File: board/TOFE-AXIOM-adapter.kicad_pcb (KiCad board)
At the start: 4 copper layers, 68.9 x 31.9 mm, 21 parts, among them CN1 C, U1 24AA01/24LC01B, U2 LM317T, U3 LM7805CT

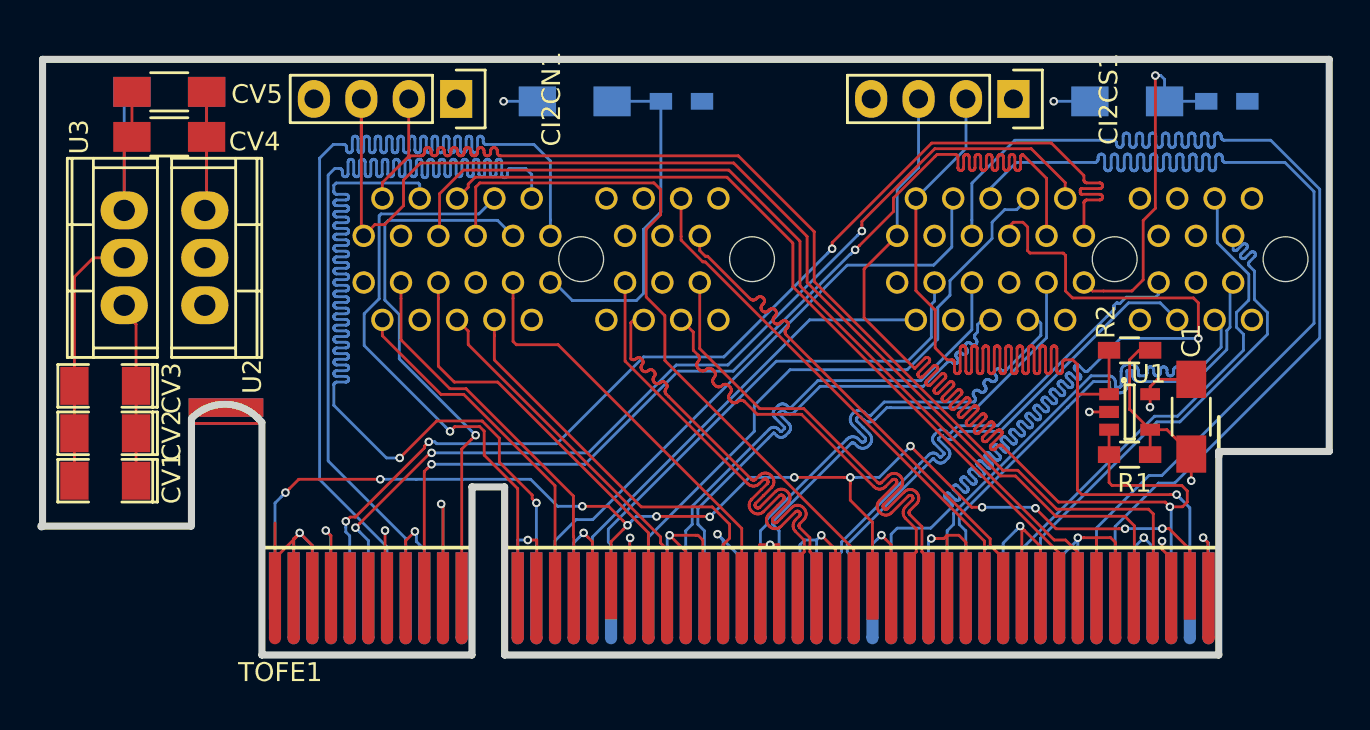
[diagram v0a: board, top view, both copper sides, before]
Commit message: Temp commit.
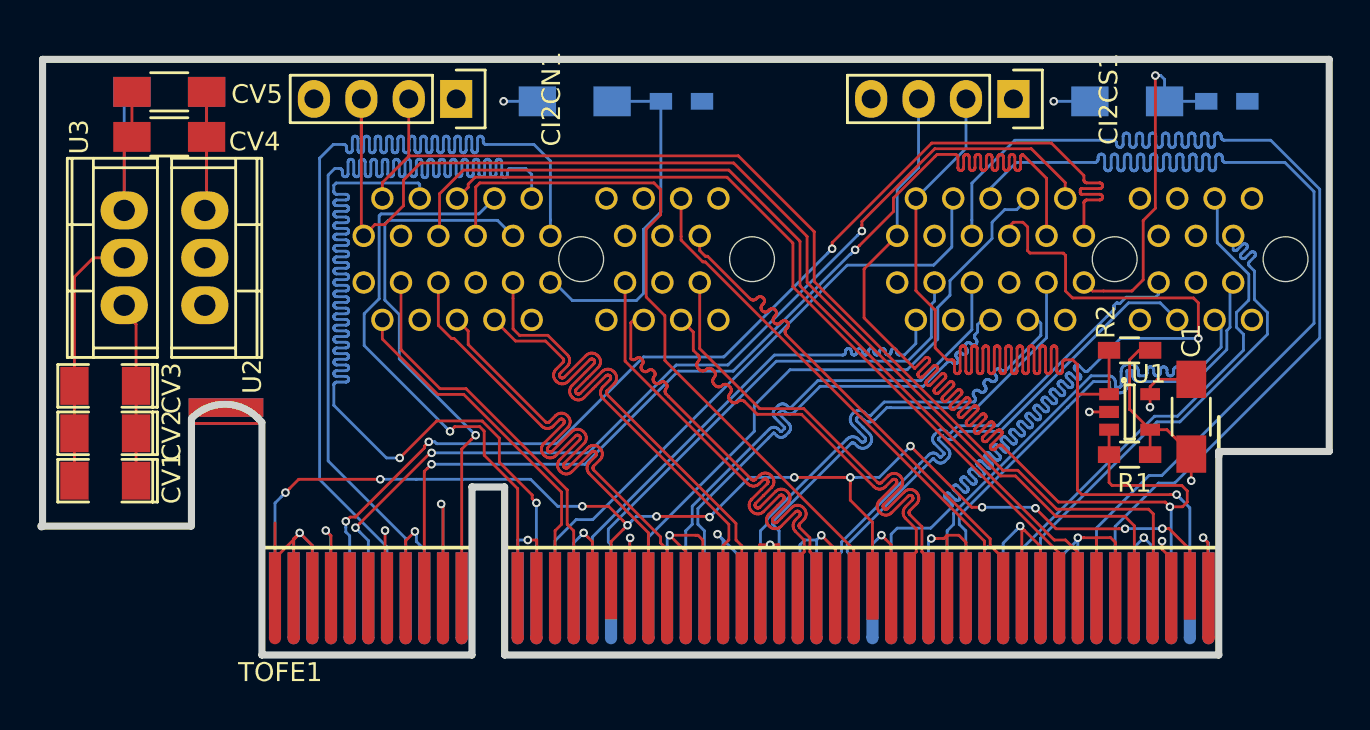
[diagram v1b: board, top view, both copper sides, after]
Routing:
- net /N_LVDS_1_N: track 21.7 -> 30.6 mm
- net /N_LVDS_1_P: track 25.1 -> 32.7 mm
- net /N_LVDS_2_N: track 25.4 -> 32.7 mm
- net /N_LVDS_2_P: track 24.6 -> 31.0 mm
- net /N_SCL: track 65.7 -> 62.1 mm
- net /S_LVDS_0_P: track 27.6 -> 30.5 mm
- net /N_SDA: track 69.5 -> 69.0 mm
